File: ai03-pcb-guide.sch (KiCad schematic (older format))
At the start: 1 part

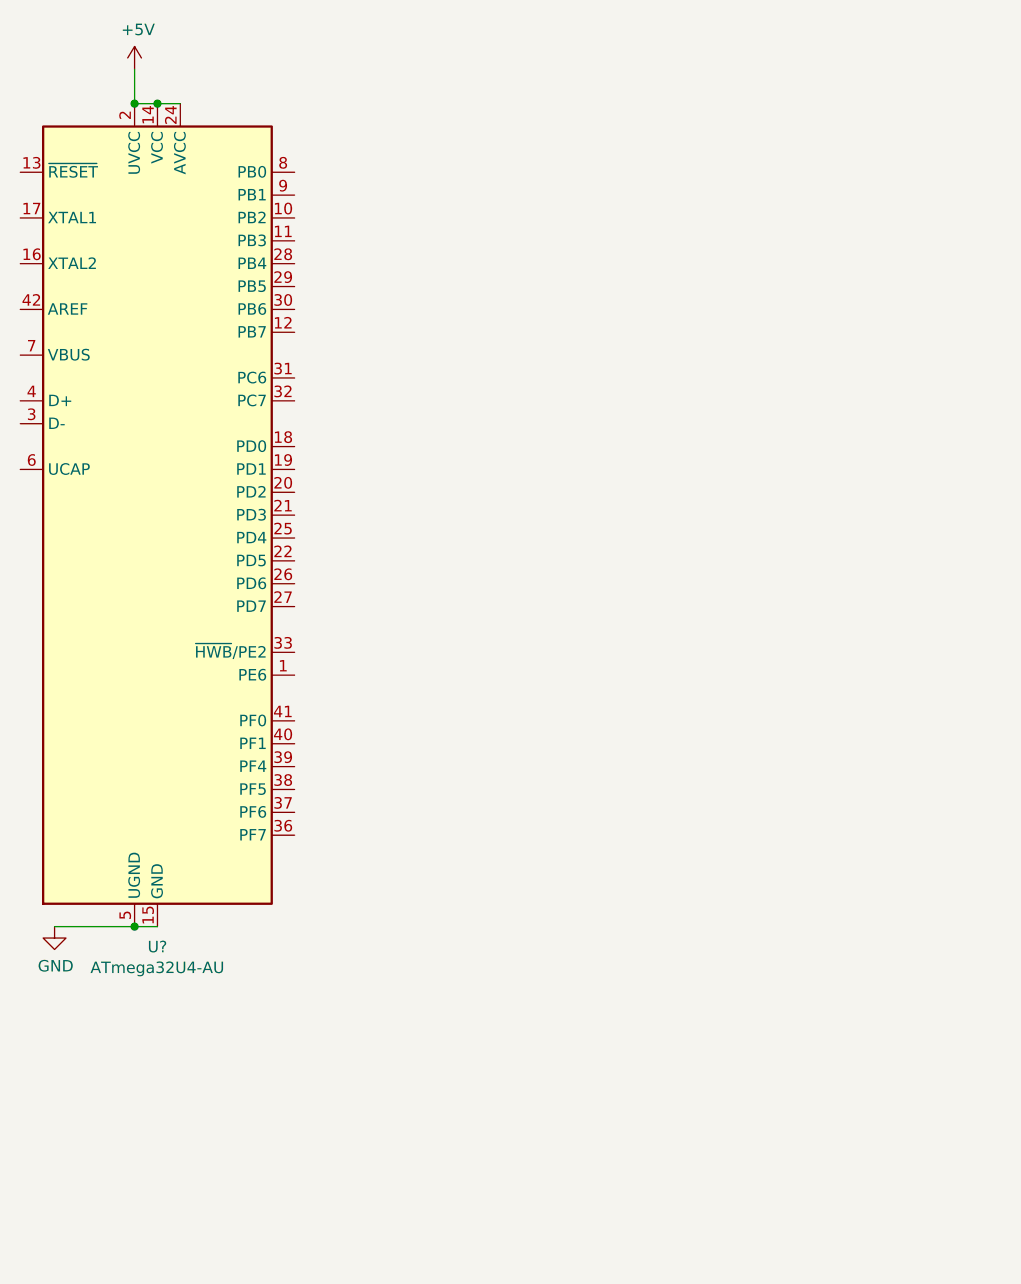
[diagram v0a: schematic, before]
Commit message: First components
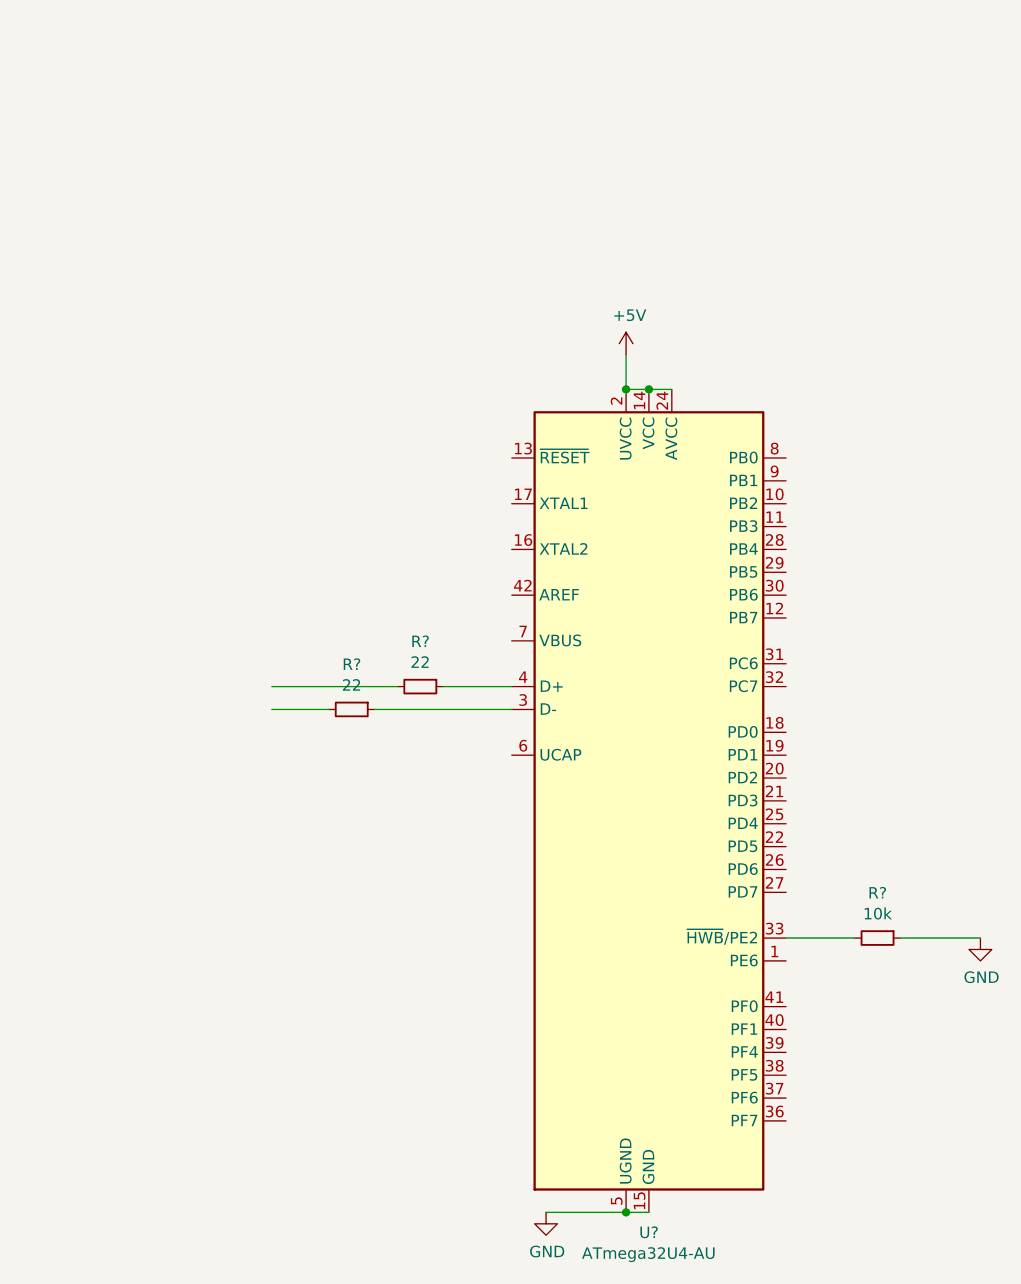
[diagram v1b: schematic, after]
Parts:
- added R?: 10k, symbol Device:R_Small
- added R? (x2): 22, symbol Device:R_Small
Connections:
- wire segments 5 -> 11
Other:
- moved on the sheet: U?
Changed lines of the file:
@@
 L power:+5V #PWR?
 U 1 1 6034AA97
-P 1250 600
-F 0 "#PWR?" H 1250 450 50  0001 C CNN
-F 1 "+5V" H 1265 773 50  0000 C CNN
-F 2 "" H 1250 600 50  0001 C CNN
-F 3 "" H 1250 600 50  0001 C CNN
-	1    1250 600
+P 3400 1850
+F 0 "#PWR?" H 3400 1700 50  0001 C CNN
+F 1 "+5V" H 3415 2023 50  0000 C CNN
+F 2 "" H 3400 1850 50  0001 C CNN
+F 3 "" H 3400 1850 50  0001 C CNN
+	1    3400 1850
 	1    0    0    -1
 $EndComp
@@
 L MCU_Microchip_ATmega:ATmega32U4-AU U?
 U 1 1 603422EB
-P 1350 2550
-F 0 "U?" H 1350 661 50  0000 C CNN
-F 1 "ATmega32U4-AU" H 1350 570 50  0000 C CNN
-F 2 "Package_QFP:TQFP-44_10x10mm_P0.8mm" H 1350 2550 50  0001 C CIN
-F 3 "http://ww1.microchip.com/downloads/en/DeviceDoc/Atmel-7766-8-bit-AVR-ATmega16U4-32U4_Datasheet.pdf" H 1350 2550 50  0001 C CNN
-	1    1350 2550
+P 3500 3800
+F 0 "U?" H 3500 1911 50  0000 C CNN
+F 1 "ATmega32U4-AU" H 3500 1820 50  0000 C CNN
+F 2 "Package_QFP:TQFP-44_10x10mm_P0.8mm" H 3500 3800 50  0001 C CIN
+F 3 "http://ww1.microchip.com/downloads/en/DeviceDoc/Atmel-7766-8-bit-AVR-ATmega16U4-32U4_Datasheet.pdf" H 3500 3800 50  0001 C CNN
+	1    3500 3800
 	1    0    0    -1
 $EndComp
 Wire Wire Line
-	1250 600  1250 750
+	3400 1850 3400 2000
 Wire Wire Line
-	1250 750  1350 750
-Connection ~ 1250 750
-Connection ~ 1350 750
+	3400 2000 3500 2000
+Connection ~ 3400 2000
+Connection ~ 3500 2000
 Wire Wire Line
-	1350 750  1450 750
+	3500 2000 3600 2000
 $Comp
 L power:GND #PWR?
 U 1 1 60353577
-P 900 4350
-F 0 "#PWR?" H 900 4100 50  0001 C CNN
-F 1 "GND" H 905 4177 50  0000 C CNN
-F 2 "" H 900 4350 50  0001 C CNN
-F 3 "" H 900 4350 50  0001 C CNN
-	1    900  4350
+P 3050 5600
+F 0 "#PWR?" H 3050 5350 50  0001 C CNN
+F 1 "GND" H 3055 5427 50  0000 C CNN
+F 2 "" H 3050 5600 50  0001 C CNN
+F 3 "" H 3050 5600 50  0001 C CNN
+	1    3050 5600
 	1    0    0    -1
 $EndComp
 Wire Wire Line
-	900  4350 1250 4350
-Connection ~ 1250 4350
+	3050 5600 3400 5600
+Connection ~ 3400 5600
 Wire Wire Line
-	1250 4350 1350 4350
+	3400 5600 3500 5600
+$Comp
+L Device:R_Small R?
+U 1 1 60354F38
+P 4500 4400
+F 0 "R?" V 4304 4400 50  0000 C CNN
+F 1 "10k" V 4395 4400 50  0000 C CNN
+F 2 "" H 4500 4400 50  0001 C CNN
+F 3 "~" H 4500 4400 50  0001 C CNN
+	1    4500 4400
+	0    1    1    0
+$EndComp
+$Comp
+L power:GND #PWR?
+U 1 1 60356495
+P 4950 4400
+F 0 "#PWR?" H 4950 4150 50  0001 C CNN
+F 1 "GND" H 4955 4227 50  0000 C CNN
+F 2 "" H 4950 4400 50  0001 C CNN
+F 3 "" H 4950 4400 50  0001 C CNN
+	1    4950 4400
+	1    0    0    -1
+$EndComp
+Wire Wire Line
+	4100 4400 4400 4400
+Wire Wire Line
+	4600 4400 4950 4400
+$Comp
+L Device:R_Small R?
+U 1 1 60365BE5
+P 2200 3400
+F 0 "R?" V 2004 3400 50  0000 C CNN
+F 1 "22" V 2095 3400 50  0000 C CNN
+F 2 "" H 2200 3400 50  0001 C CNN
+F 3 "~" H 2200 3400 50  0001 C CNN
+	1    2200 3400
+	0    1    1    0
+$EndComp
+Wire Wire Line
+	2900 3300 2600 3300
+Wire Wire Line
+	2400 3300 1850 3300
+Wire Wire Line
+	2100 3400 1850 3400
+Wire Wire Line
+	2900 3400 2300 3400
+$Comp
+L Device:R_Small R?
+U 1 1 6036534E
+P 2500 3300
+F 0 "R?" V 2304 3300 50  0000 C CNN
+F 1 "22" V 2395 3300 50  0000 C CNN
+F 2 "" H 2500 3300 50  0001 C CNN
+F 3 "~" H 2500 3300 50  0001 C CNN
+	1    2500 3300
+	0    1    1    0
+$EndComp
 $EndSCHEMATC

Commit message: Complete MCU
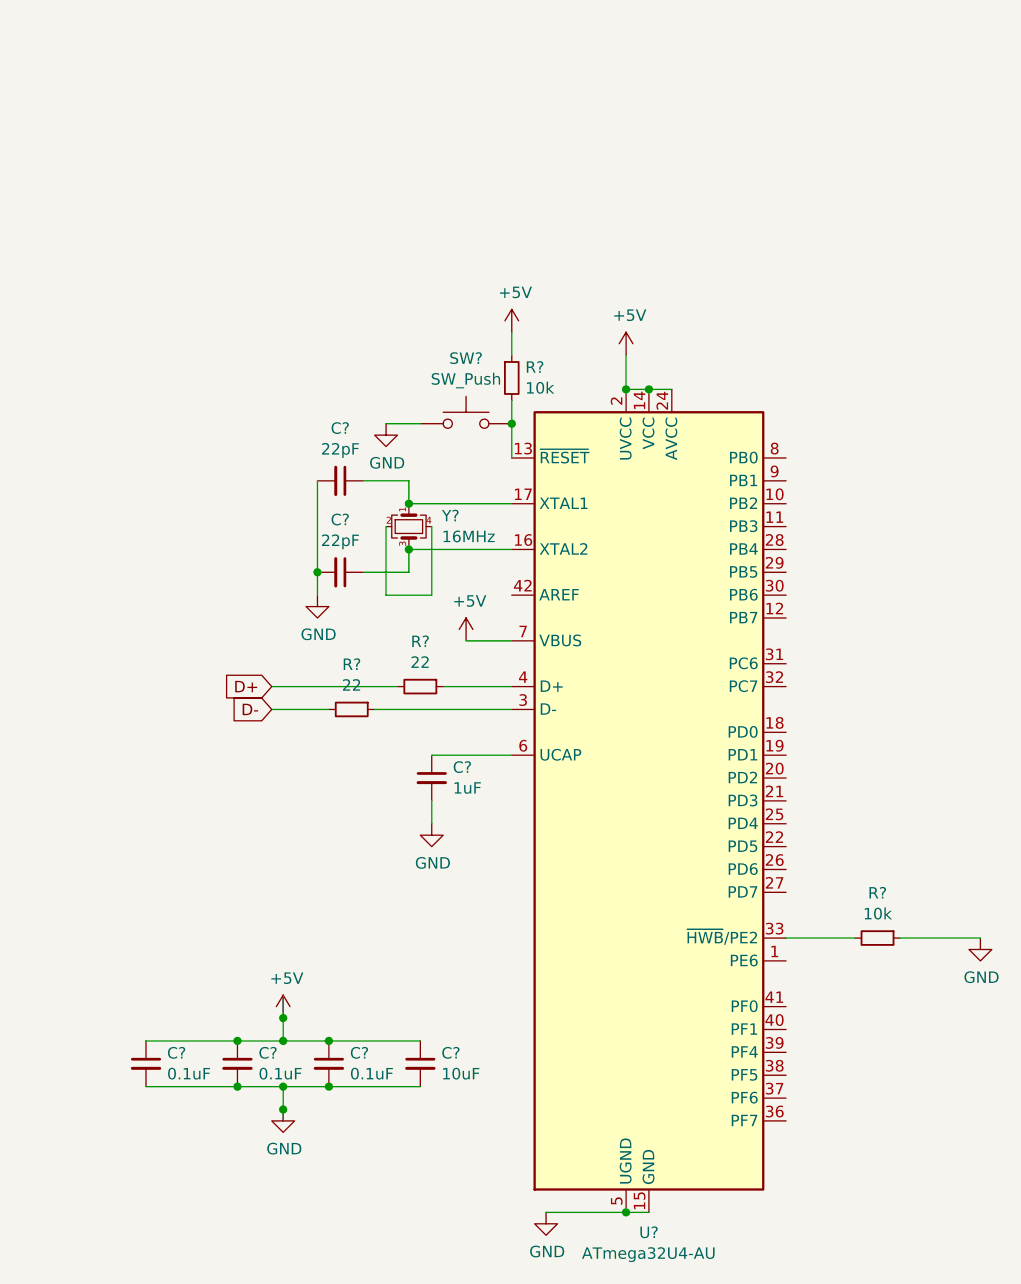
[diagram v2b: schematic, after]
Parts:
- added C? (x3): 0.1uF, symbol Device:C_Small
- added C?: 10uF, symbol Device:C_Small
- added C? (x2): 22pF, symbol Device:C_Small
- added C?: 1uF, symbol Device:C_Small
- added R?: 10k, symbol Device:R_Small
- added SW?: SW_Push, symbol Switch:SW_Push
- added Y?: 16MHz, symbol Device:Crystal_GND24_Small
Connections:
- net labels added: D+, D-
- wire segments 11 -> 41
